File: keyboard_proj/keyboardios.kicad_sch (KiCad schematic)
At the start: 23 parts

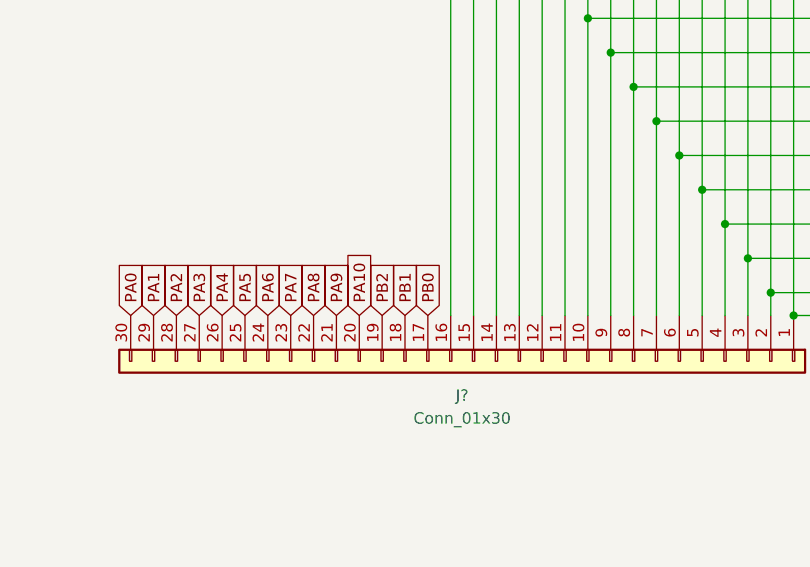
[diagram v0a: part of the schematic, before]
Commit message: Tous les schematics vérifiés 1x
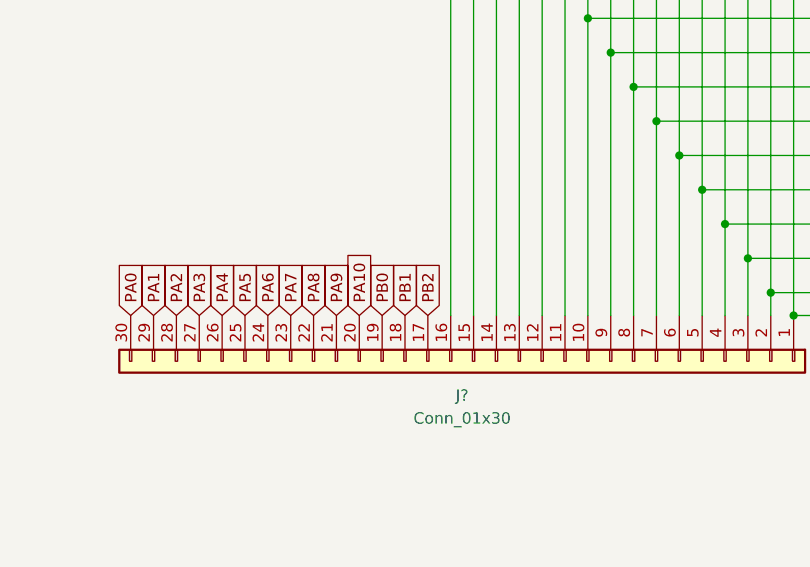
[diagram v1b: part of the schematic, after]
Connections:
- net PB0: now also J?.19 (Pin_19); no longer J?.17 (Pin_17)
- net PB2: now also J?.17 (Pin_17); no longer J?.19 (Pin_19)
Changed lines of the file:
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@@
     )
   )
-  (global_label "PB0" (shape input) (at 154.94 129.54 90) (fields_autoplaced)
+  (global_label "PB0" (shape input) (at 149.86 129.54 90) (fields_autoplaced)
     (effects (font (size 1.27 1.27)) (justify left))
-    (property "Intersheet References" "${INTERSHEET_REFS}" (id 0) (at 155.0194 123.3774 90)
+    (property "Intersheet References" "${INTERSHEET_REFS}" (id 0) (at 149.9394 123.3774 90)
       (effects (font (size 1.27 1.27)) (justify left) hide)
     )
@@
     )
   )
-  (global_label "PB2" (shape input) (at 149.86 129.54 90) (fields_autoplaced)
+  (global_label "PB2" (shape input) (at 154.94 129.54 90) (fields_autoplaced)
     (effects (font (size 1.27 1.27)) (justify left))
-    (property "Intersheet References" "${INTERSHEET_REFS}" (id 0) (at 149.9394 123.3774 90)
+    (property "Intersheet References" "${INTERSHEET_REFS}" (id 0) (at 155.0194 123.3774 90)
       (effects (font (size 1.27 1.27)) (justify left) hide)
     )
